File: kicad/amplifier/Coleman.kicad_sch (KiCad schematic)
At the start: 0 parts

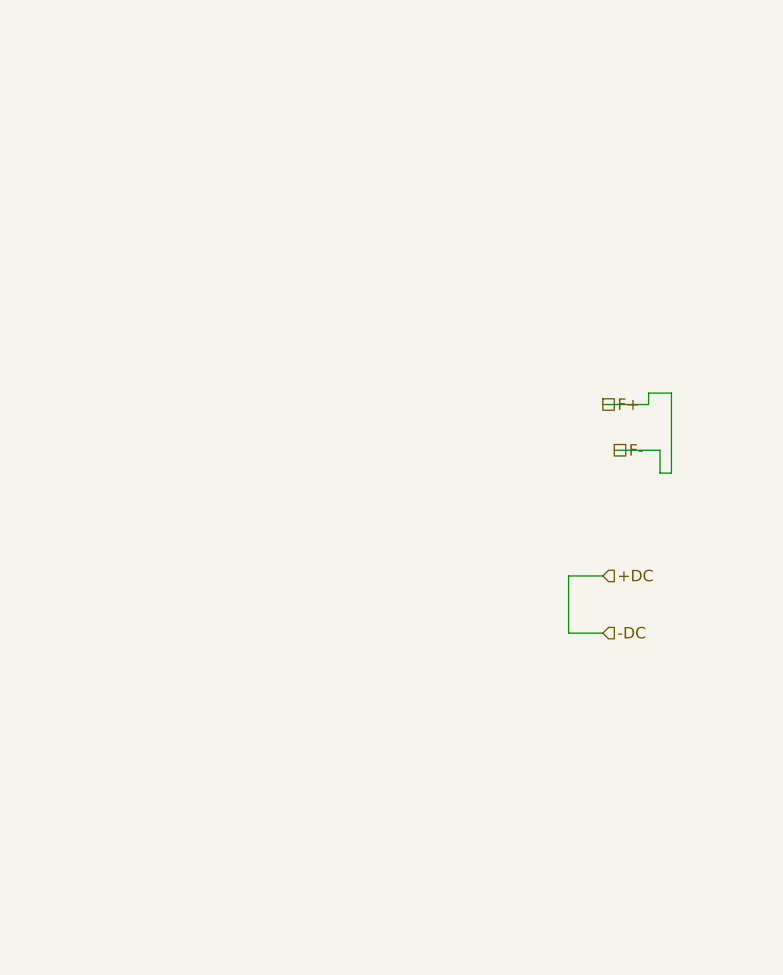
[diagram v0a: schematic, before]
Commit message: coleman
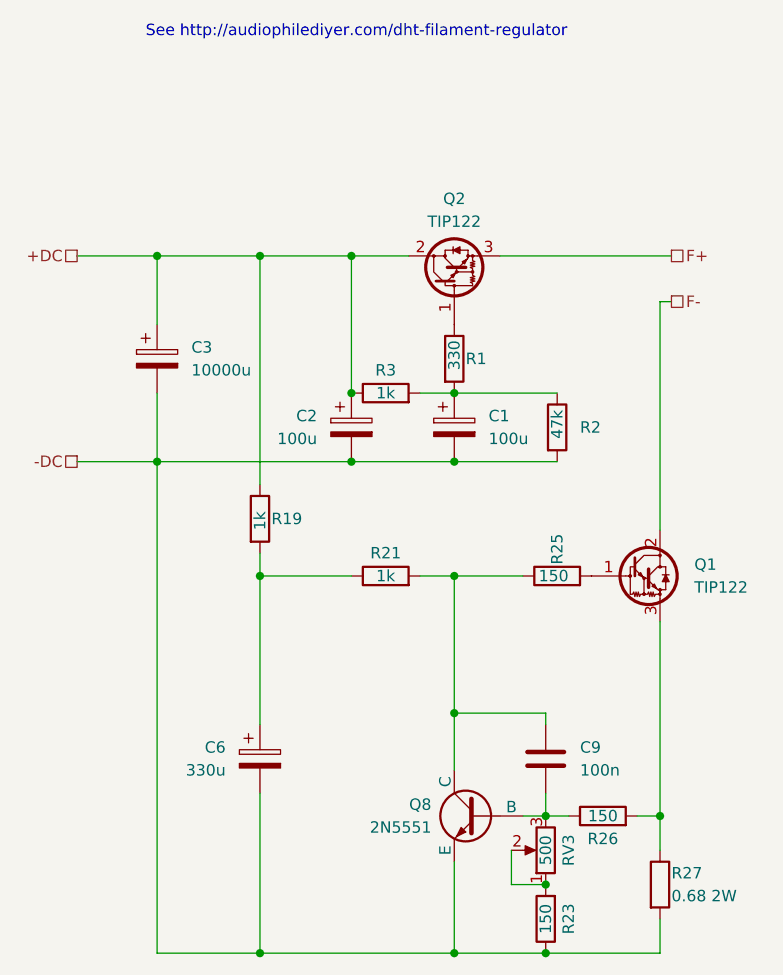
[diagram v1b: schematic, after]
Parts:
- added C1, C2: 100u, symbol Device:C_Polarized
- added C3: 10000u, Capacitor_THT:CP_Radial_D25.0mm_P10.00mm_SnapIn, symbol Device:C_Polarized
- added C6: 330u, symbol Device:C_Polarized
- added C9: 100n, symbol Device:C
- added Q1, Q2: TIP122, Package_TO_SOT_THT:TO-220-3_Vertical, symbol Transistor_BJT:TIP122
- added Q8: 2N5551, symbol Simulation_SPICE:NPN
- added R1: 330, symbol Device:R
- added R19, R21, R3: 1k, symbol Device:R
- added R2: 47k, symbol Device:R
- added R23, R25, R26: 150, symbol Device:R
- added R27: 0.68 2W, symbol Device:R
- added RV3: 500, symbol Device:R_Potentiometer
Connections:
- net +DC: now also C2.1, C3.1, Q2.2 (C), R19.1, R3.1
- net F+: now also Q2.3 (E)
- new net: Q2.1 (B), R1.1
- new net: C1.1, R1.2, R2.1, R3.2
- new net: C9.1, Q8.1 (C), R21.2, R25.1
- new net: C9.2, Q8.2 (B), R26.1, RV3.3
- new net: Q1.3 (E), R26.2, R27.1
- new net: C6.1, R19.2, R21.1
- new net: R23.2, RV3.1, RV3.2
- new net: Q1.1 (B), R25.2
- new net -DC: C1.2, C2.2, C3.2, C6.2, Q8.3 (E), R2.2, R23.1, R27.2
- new net F-: Q1.2 (C)
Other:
- note added: "See http://audiophilediyer.com/dht-filament-regulator"

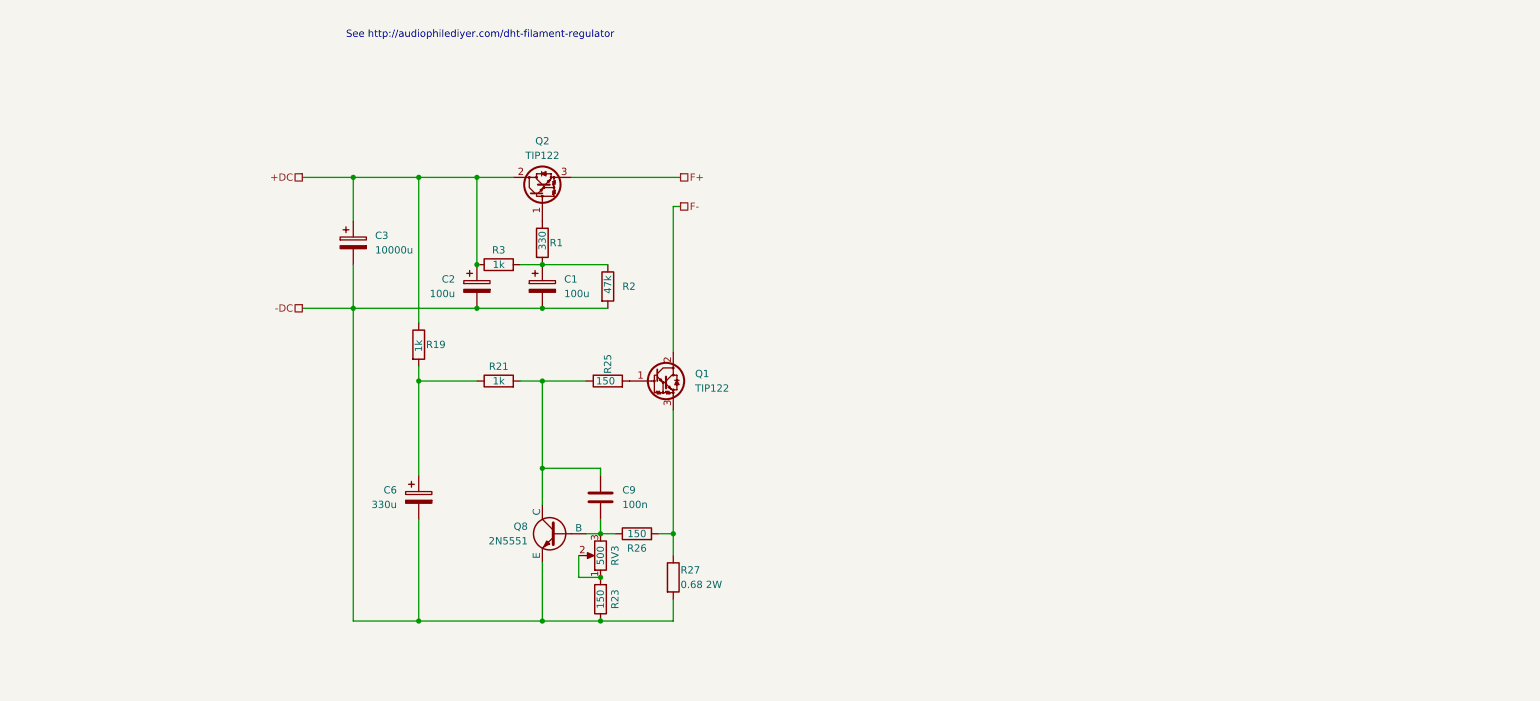
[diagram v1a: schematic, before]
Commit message: 801 filament supply
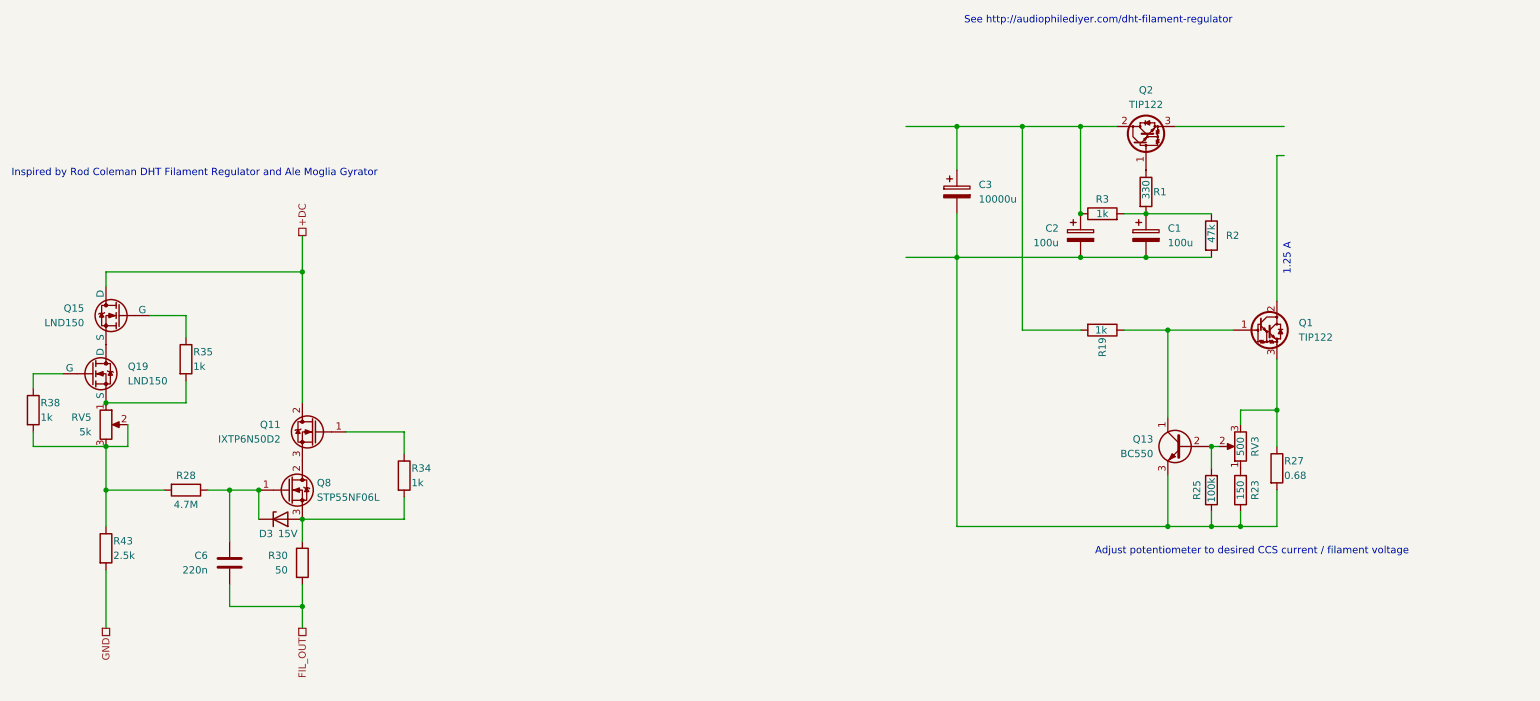
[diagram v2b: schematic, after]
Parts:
- removed C6: 330u, symbol Device:C_Polarized
- removed C9: 100n, symbol Device:C
- removed Q8: 2N5551, symbol Simulation_SPICE:NPN
- removed R21: 1k, symbol Device:R
- removed R26: 150, symbol Device:R
- added C6: 220n, Capacitor_THT:C_Rect_L26.5mm_W10.5mm_P22.50mm_MKS4, symbol Device:C
- added D3: 15V, Diode_THT:D_DO-34_SOD68_P7.62mm_Horizontal, symbol Device:D_Zener
- added Q11: IXTP6N50D2, Package_TO_SOT_THT:TO-220-3_Vertical, symbol stax_ccs:10M90S
- added Q13: BC550, Package_TO_SOT_THT:TO-92_Inline, symbol Transistor_BJT:BC550
- added Q15, Q19: LND150, symbol Simulation_SPICE:NMOS
- added Q8: STP55NF06L, Package_TO_SOT_THT:TO-220-3_Vertical, symbol Transistor_FET_Other:DN2540N5-G
- added R28: 4.7M, Resistor_THT:R_Axial_DIN0207_L6.3mm_D2.5mm_P10.16mm_Horizontal, symbol Device:R
- added R30: 50, Resistor_THT:R_Axial_DIN0207_L6.3mm_D2.5mm_P10.16mm_Horizontal, symbol Device:R
- added R34, R35, R38: 1k, Resistor_THT:R_Axial_DIN0207_L6.3mm_D2.5mm_P10.16mm_Horizontal, symbol Device:R
- added R43: 2.5k, Resistor_THT:R_Axial_DIN0207_L6.3mm_D2.5mm_P10.16mm_Horizontal, symbol Device:R
- added RV5: 5k, symbol Device:R_Potentiometer
- R25: value 150 -> 100k
- R27: value 0.68 2W -> 0.68
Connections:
- net -DC is gone; now on an unnamed net: C1.2, C2.2, C3.2, R2.2, R23.1, R27.2
- net +DC: now also Q11.2 (P), Q15.1 (D); no longer C2.1, C3.1, Q2.2 (C), R19.1, R3.1
- net at R25.1: now also Q13.3 (E)
- net at RV3.3: now also Q1.3 (E), R27.1
- net at R19.2: now also C2.1, C3.1, Q2.2 (C), R3.1
- net at R23.2, RV3.1: no longer RV3.2
- net at R25.2: now also RV3.2, Q13.2 (B); no longer Q1.1 (B)
- net F+: no longer names the net of Q2.3 (E)
- net F-: no longer names the net of Q1.2 (C)
- new net: C6.1, D3.1 (K), Q8.1 (G), R28.1
- new net: D3.2 (A), Q8.3 (S), R30.1, R34.2
- new net: Q15.2 (G), R35.1
- new net: Q15.3 (S), Q19.1 (D)
- new net: Q19.2 (G), R38.1
- new net: Q19.3 (S), R35.2, RV5.1
- new net: R28.2, R38.2, R43.1, RV5.2, RV5.3
- new net: Q1.1 (B), Q13.1 (C), R19.1
- new net: Q11.3 (N), Q8.2 (D)
- new net: Q11.1 (G), R34.1
- new net FIL_OUT: C6.2, R30.2
- new net GND: R43.2
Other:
- note added: "1.25 A"
- note added: "Adjust potentiometer to desired CCS current / filament voltage"
- note added: "Inspired by Rod Coleman DHT Filament Regulator and Ale Moglia Gyrator"
- moved on the sheet: C1, C2, C3, Q1, Q2, R1, R2, R23, R27, R3, RV3
